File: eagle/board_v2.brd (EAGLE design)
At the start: 100 x 62.9 mm, 35 parts, among them J1 RJ11-4X, J2 RJ11-4X, Q1 BD140, Q10 BD140, Q11 BD140, Q12 BD140, Q13 BD140, Q14 BD140, Q15 BD140, Q2 BD140, Q3 BD140, Q4 BD140, Q5 BD140, Q6 BD140, Q7 BD140, Q8 BD140, Q9 BD140, X1 RJ45-8X, X2 RJ45-8X, X3 RJ45-8X, X4 RJ45-8X, X5 RJ45-8X, X6 RJ45-8X

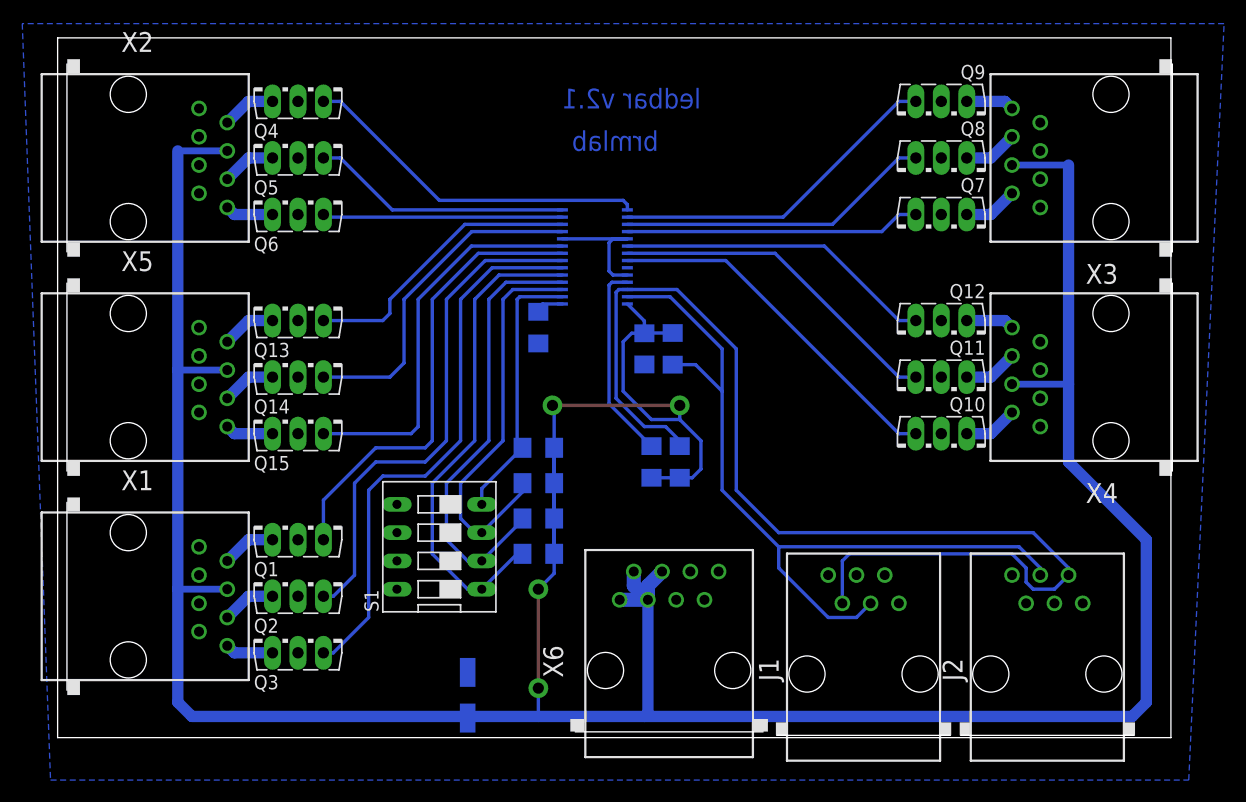
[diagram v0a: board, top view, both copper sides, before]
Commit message: board v2.2
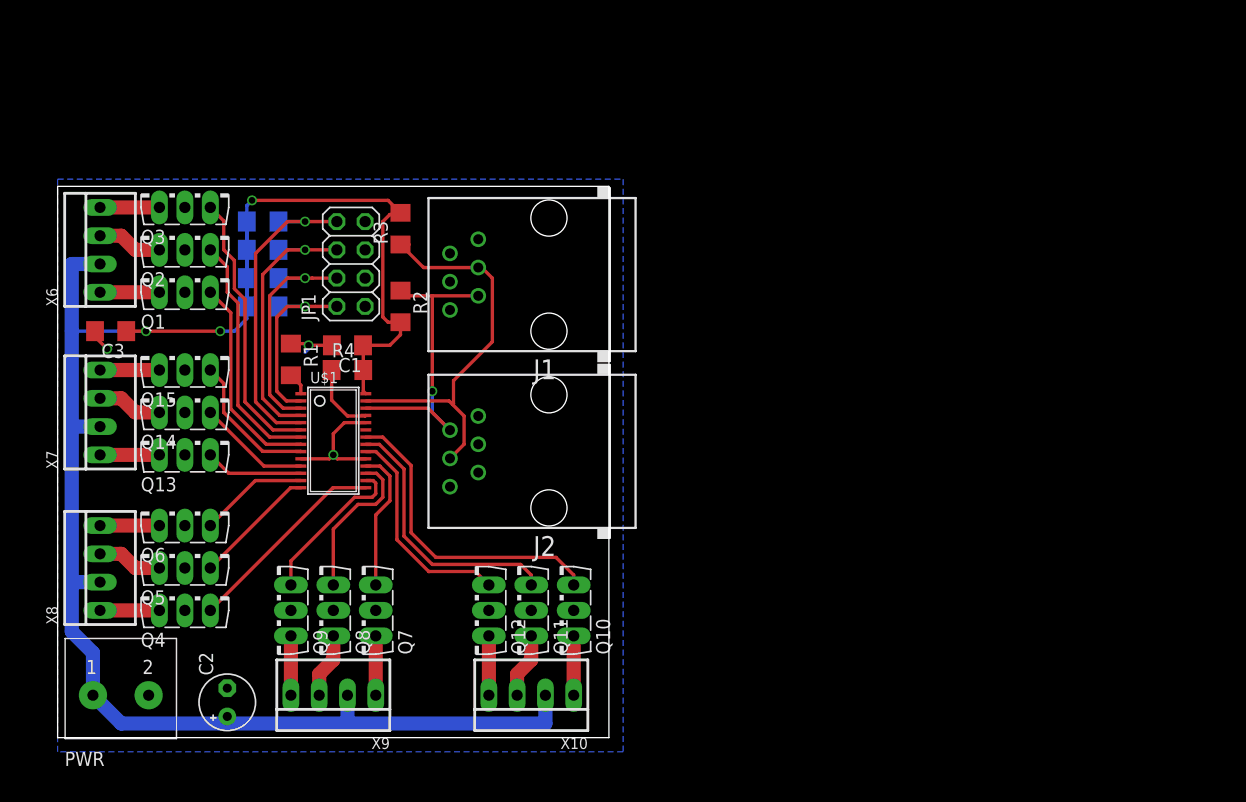
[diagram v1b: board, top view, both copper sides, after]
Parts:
- removed S1: (no value), switch-dil:DS-04
- removed X1, X2, X3, X4, X5: RJ45-8X, con-tycoelectronics:RJ45-NO-SHIELD
- added C3: 1u, resistor:C1206
- added JP1: (no value), pinhead:2X04
- added PWR: ARK210/2EX, con-brm:ARK210/2EX
- added X10, X7, X8, X9: 22-23-2041, con-molex:22-23-2041
- C2: device resistor:PANASONIC_C -> resistor:E2,5-5
- R4: value 10k -> 4k7
- X6: value RJ45-8X -> 22-23-2041; device con-tycoelectronics:RJ45-NO-SHIELD -> con-molex:22-23-2041
- moved Q9 74.4 mm to (19.7, 11.4), turned to 90 degrees
- moved Q8 68.4 mm to (23.5, 11.4), turned to 90 degrees
- moved X6 63.6 mm to (3.81, 43.8), turned to 90 degrees
- moved Q7 62.3 mm to (27.3, 11.4), turned to 90 degrees
- moved J2 49.0 mm to (44.1, 25.7), turned to 90 degrees
- moved Q12 48.7 mm to (37.5, 11.4), turned to 90 degrees
- moved Q4 46.8 mm to (11.4, 12.7)
- moved J1 45.7 mm to (44.1, 41.6), turned to 90 degrees
- moved Q11 42.9 mm to (41.3, 11.4), turned to 90 degrees
- moved Q3 41.3 mm to (11.4, 48.9)
- moved R5 38.8 mm to (18.4, 46.4), turned to 180 degrees
- moved Q5 38.2 mm to (11.4, 16.5)
- moved Q10 37.3 mm to (45.1, 11.4), turned to 90 degrees
- moved R6 34.6 mm to (18.4, 43.8), turned to 180 degrees
- moved Q2 32.7 mm to (11.4, 45.1)
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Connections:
- net +5V: now also C3.1, PWR.P$1, X10.2, X7.2, X8.2, X9.2; no longer X1.4, X2.4, X3.4, X4.4, X5.4, X6.1, X6.3, X6.4
- net GND: now also C3.2, JP1.1, JP1.3, JP1.5, JP1.7, PWR.P$2; no longer S1.5, S1.6, S1.7, S1.8, X6.5, X6.6, X6.7, X6.8
- net N$1: now also X6.1; no longer X1.2
- net N$10: now also X10.1; no longer X4.2
- net N$11: now also X10.3; no longer X4.6
- net N$12: now also X10.4; no longer X4.8
- net N$13: now also X7.1; no longer X5.2
- net N$14: now also X7.3; no longer X5.6
- net N$15: now also X7.4; no longer X5.8
- net N$17: now also JP1.2; no longer S1.4
- net N$18: now also JP1.4; no longer S1.3
- net N$19: now also JP1.6; no longer S1.2
- net N$2: now also X6.3; no longer X1.6
- net N$20: now also JP1.8; no longer S1.1
- net N$3: now also X6.4; no longer X1.8
- net N$4: now also X8.1; no longer X2.2
- net N$5: now also X8.3; no longer X2.6
- net N$6: now also X8.4; no longer X2.8
- net N$7: now also X9.1; no longer X3.2
- net N$8: now also X9.3; no longer X3.6
- net N$9: now also X9.4; no longer X3.8
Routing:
- net +5V: track 312.3 -> 167.3 mm, vias 4 -> 3
- net N$37: track 103.6 -> 28.5 mm, vias 0 -> 1
- net N$38: track 73.2 -> 36.8 mm
- net N$22: track 49.9 -> 24.8 mm
- net N$23: track 46.2 -> 21.8 mm
- net N$24: track 41.6 -> 18.8 mm
- net N$16: track 35.1 -> 12.7 mm
- net N$25: track 30.2 -> 10.1 mm
- net N$26: track 25.8 -> 8.82 mm
- net N$30: track 30.2 -> 14.2 mm
- net N$20: track 44.0 -> 29.0 mm, vias 0 -> 1
- net N$19: track 39.7 -> 25.2 mm, vias 0 -> 1
- net N$31: track 28.4 -> 14.0 mm
- net N$18: track 35.4 -> 21.3 mm, vias 0 -> 1
- net N$32: track 26.5 -> 12.8 mm
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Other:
- board size 100 x 62.9 mm -> 49.5 x 49.5 mm
- board text removed: "C1"
- board text removed: "C2"
- board text removed: "J1"
- board text removed: "J2"
- board text removed: "Q1"
- board text removed: "Q10"
- board text removed: "Q11"
- board text removed: "Q12"
- board text removed: "Q13"
- board text removed: "Q14"
- board text removed: "Q15"
- board text removed: "Q2"
- board text removed: "Q3"
- board text removed: "Q4"
- board text removed: "Q5"
- board text removed: "Q6"
- board text removed: "Q7"
- board text removed: "Q8"
- board text removed: "Q9"
- board text removed: "R1"
- board text removed: "R2"
- board text removed: "R3"
- board text removed: "R4"
- board text removed: "R5"
- board text removed: "R6"
- board text removed: "R7"
- board text removed: "R8"
- board text removed: "S1"
- board text removed: "U$1"
- board text removed: "X2"
- board text removed: "X3"
- board text removed: "X4"
- board text removed: "X6"
- board text removed: "brmlab"
- board text removed: "ledbar v2.1"
